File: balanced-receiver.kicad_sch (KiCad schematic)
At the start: 40 parts, among them J1 Barrel_Jack_Switch, J2 Screw_Terminal_01x02, J3 Screw_Terminal_01x02, J4 Screw_Terminal_01x03, Q1 Q_PMOS_GDS, U1 LM1117DT-3.3, U2 LM1117DT-1.8, U3 TPS62932, U4 LM2776

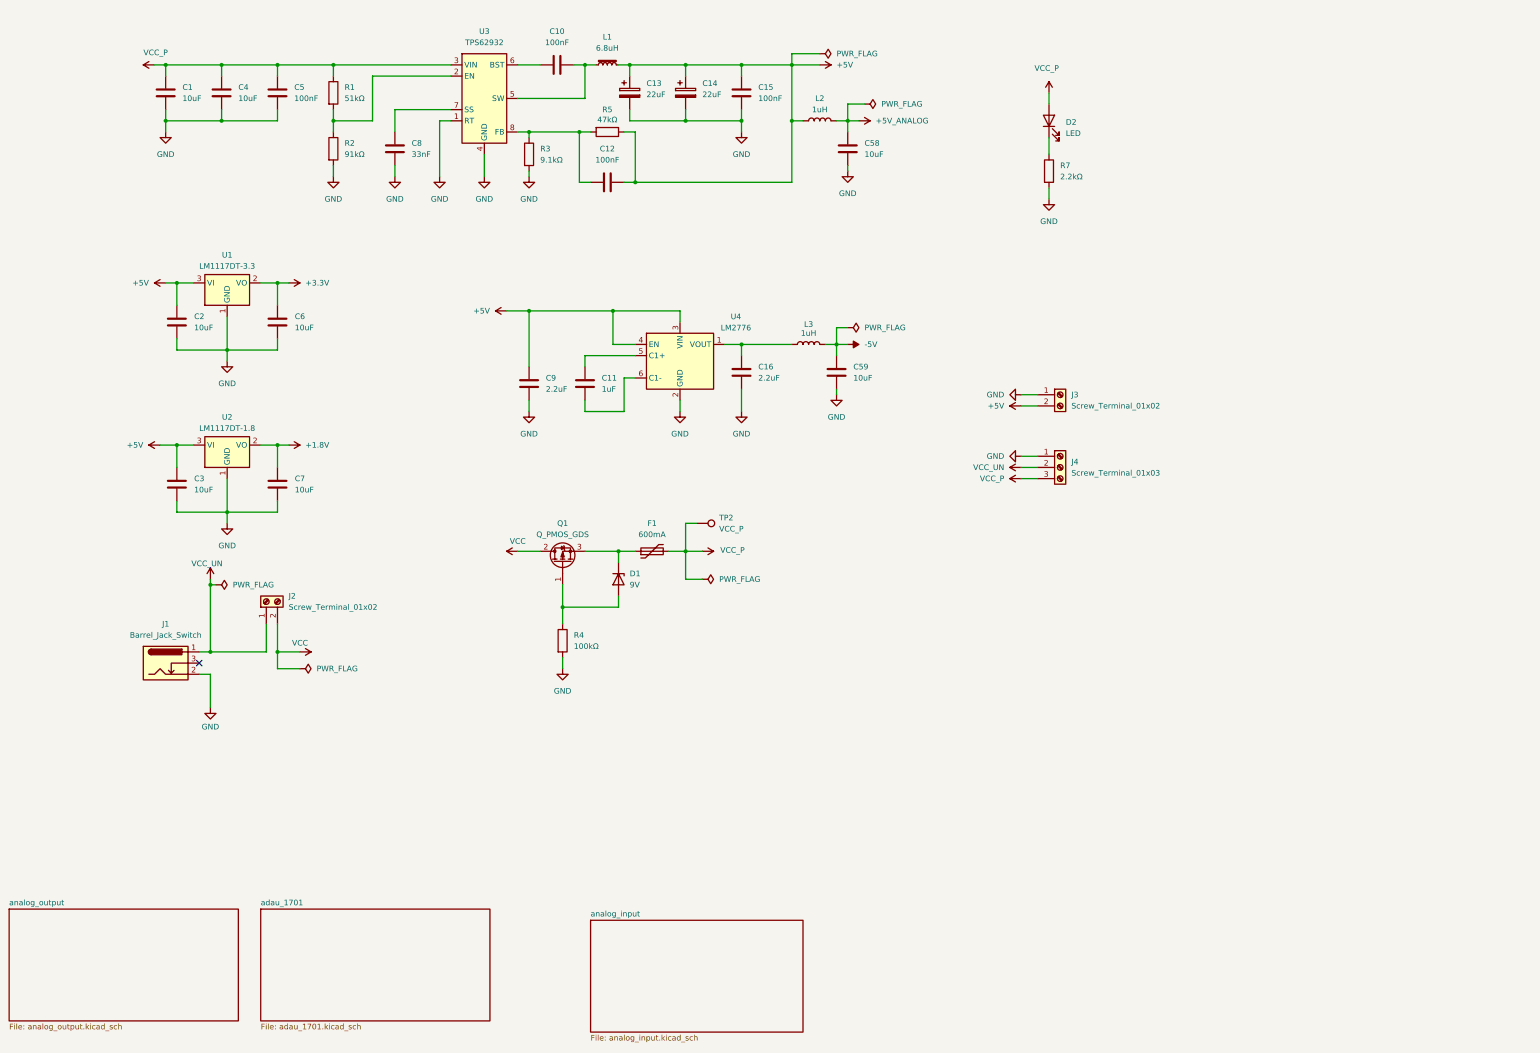
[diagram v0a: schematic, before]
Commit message: WIP
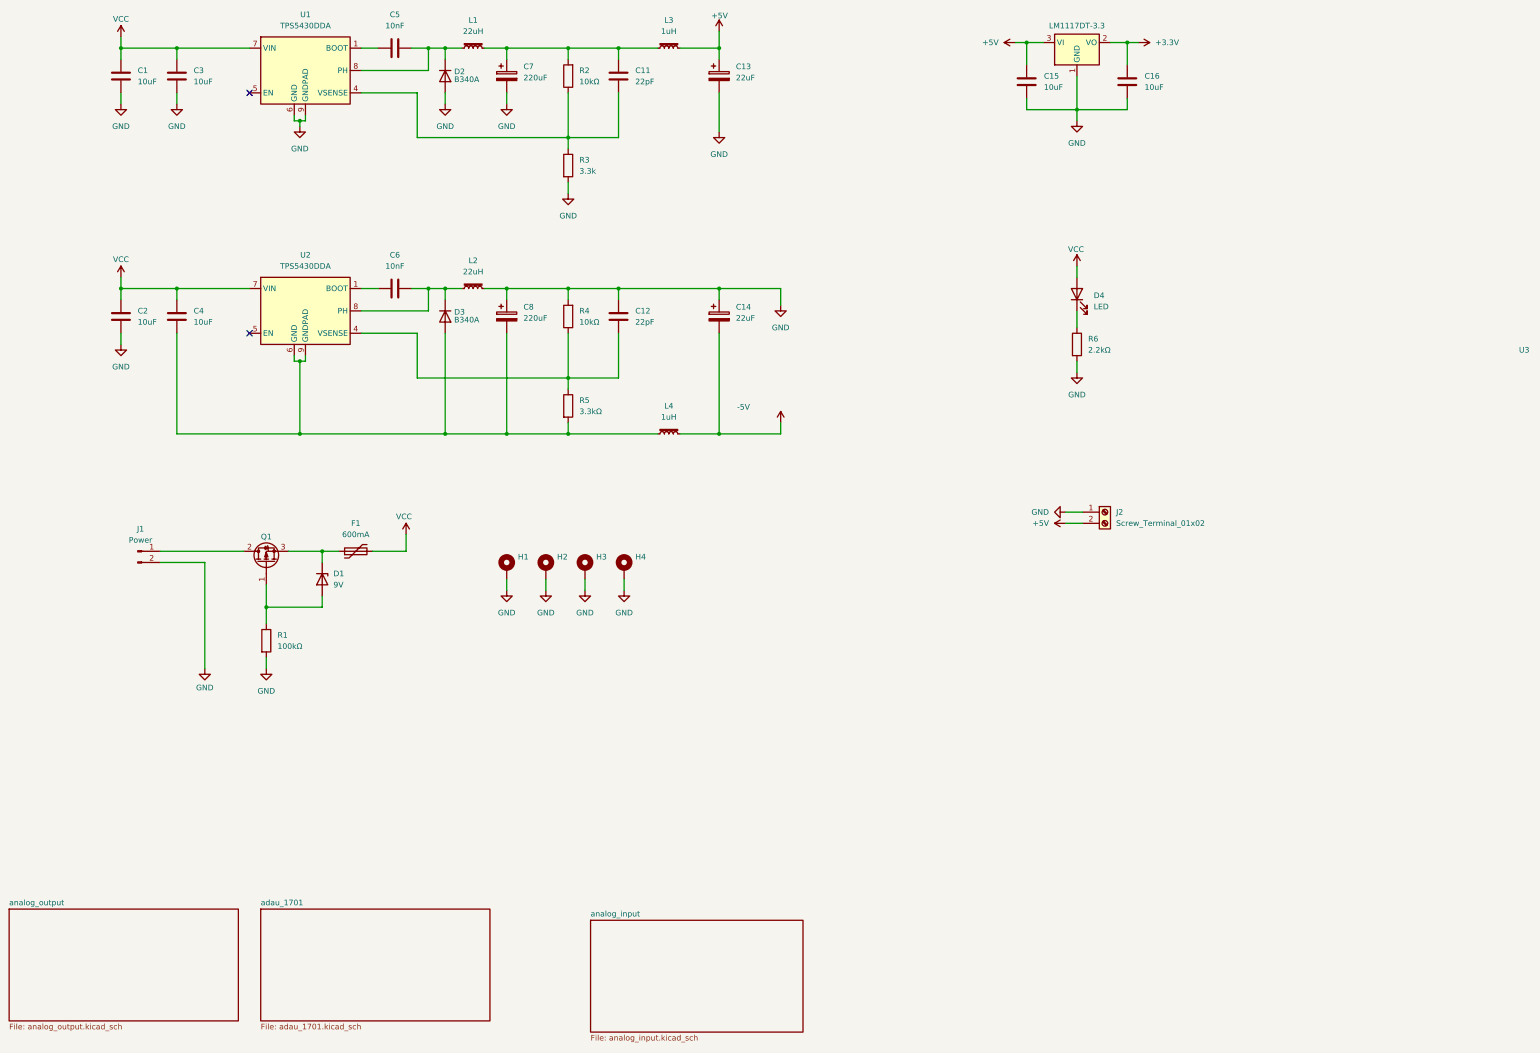
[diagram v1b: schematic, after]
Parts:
- removed C10, C15: 100nF, Capacitor_SMD:C_0805_2012Metric_Pad1.18x1.45mm_HandSolder, symbol Device:C
- removed C16, C9: 2.2uF, Capacitor_SMD:C_0805_2012Metric_Pad1.18x1.45mm_HandSolder, symbol Device:C
- removed C58, C59, C7: 10uF, Capacitor_SMD:C_0805_2012Metric_Pad1.18x1.45mm_HandSolder, symbol Device:C
- removed C8: 33nF, Capacitor_SMD:C_0805_2012Metric_Pad1.18x1.45mm_HandSolder, symbol Device:C
- removed J1: Barrel_Jack_Switch, balanced-receiver:BarrelJack_GCT_DCJ200-10-A_Horizontal, symbol Connector:Barrel_Jack_Switch
- removed J2: Screw_Terminal_01x02, balanced-receiver:TerminalBlock_Phoenix_MPT-0,5-2-2.54_1x02_P2.54mm_Horizontal, symbol Connector:Screw_Terminal_01x02
- removed J4: Screw_Terminal_01x03, balanced-receiver:TerminalBlock_1x03_P7.50mm_Horizontal, symbol Connector:Screw_Terminal_01x03
- removed L2, L3: 1uH, Inductor_SMD:L_0805_2012Metric_Pad1.05x1.20mm_HandSolder, symbol Device:L
- removed R1: 51kΩ, Resistor_SMD:R_0805_2012Metric_Pad1.20x1.40mm_HandSolder, symbol Device:R
- removed TP2: VCC_P, TestPoint:TestPoint_Pad_D1.0mm, symbol Connector:TestPoint
- removed U2: LM1117DT-1.8, Package_TO_SOT_SMD:SOT-223-3_TabPin2, symbol Regulator_Linear:LM1117DT-1.8
- removed U3: TPS62932, balanced-receiver:SOT-583-8, symbol Regulator_Switching:TPS62932
- removed U4: LM2776, Package_TO_SOT_SMD:SOT-23-6_Handsoldering, symbol Regulator_SwitchedCapacitor:LM2776
- added C2: 10uF, Capacitor_SMD:C_0805_2012Metric_Pad1.18x1.45mm_HandSolder, symbol Device:C
- added C6: 10nF, Capacitor_SMD:C_0805_2012Metric_Pad1.18x1.45mm_HandSolder, symbol Device:C
- added C7, C8: 220uF, Capacitor_SMD:CP_Elec_6.3x7.7, symbol Device:C_Polarized
- added D2, D3: B340A, Diode_SMD:D_SMA_Handsoldering, symbol Device:D
- added H1, H2, H3, H4: MountingHole_Pad_MP, MountingHole_2.2mm_M2_DIN965_Pad_TopBottom, symbol Mechanical:MountingHole_Pad_MP
- added J1: Power, Connector_JST:JST_XH_B2B-XH-A_1x02_P2.50mm_Vertical, symbol Connector:Conn_01x02_Pin
- added L2: 22uH, Inductor_SMD:L_APV_ANR6028, symbol Device:L_Iron_Small
- added L3, L4: 1uH, Inductor_SMD:L_APV_APH0420, symbol Device:L_Iron_Small
- added R4: 10kΩ, Resistor_SMD:R_0805_2012Metric_Pad1.20x1.40mm_HandSolder, symbol Device:R
- added U1, U2: TPS5430DDA, Package_SO:TI_SO-PowerPAD-8, symbol Regulator_Switching:TPS5430DDA
- C11: value 1uF -> 22pF
- C12: value 100nF -> 22pF
- C5: value 100nF -> 10nF
- L1: value 6.8uH -> 22uH; footprint Inductor_SMD:L_APV_APH0530 -> Inductor_SMD:L_APV_ANR6028
- R2: value 91kΩ -> 10kΩ
- R3: value 9.1kΩ -> 3.3k
- R5: value 47kΩ -> 3.3kΩ
- renumbered C2 to C15, C6 to C16, D2 to D4, J3 to J2, R4 to R1, R7 to R6, U1 to U3
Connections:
- net +5V: now also L3.2; no longer C12.2, C14.1, C3.2, L1.2, R5.1
- net -5V: now also C14.2, L4.2
- net GND: now also C12.1, C14.1, C3.2, C2.2, C7.2, C8.1, D2.2 (A), H1.MP, H2.MP, H3.MP, H4.MP, J1.2 (Pin_2), L2.2, R4.2, U1.6 (GND), U1.9 (GNDPAD); no longer C14.2, C3.1, C4.2, C5.2, R2.2
- net VCC: now also C1.1, C3.1, C4.1, D4.2 (A), F1.2, C2.1, U1.7 (VIN), U2.7 (VIN); no longer Q1.2 (D)
- net at R2.1: now also C11.2, R3.1, U1.4 (VSENSE)
- net at L1.1: now also C5.2, D2.1 (K), U1.8 (PH)
- net at C11.1: now also L1.2, R2.2, C7.1, L3.1
- removed net VCC_P: C1.1, C4.1, C5.1, D4.2 (A), F1.2
- new net: C12.2, R4.1, R5.1, U2.4 (VSENSE)
- new net: C4.2, C8.2, D3.2 (A), L4.1, R5.2, U2.6 (GND), U2.9 (GNDPAD)
- new net: J1.1 (Pin_1), Q1.2 (D)
- new net: C6.1, U2.1 (BOOT)
- new net: C6.2, D3.1 (K), L2.1, U2.8 (PH)
- new net: C5.1, U1.1 (BOOT)
- no-connect marks 1 -> 2
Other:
- moved on the sheet: C15, C16, D1, D4, F1, J2, Q1, R1, R6, U3
